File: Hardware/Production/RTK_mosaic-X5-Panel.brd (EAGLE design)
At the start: 151.8 x 101.6 mm, 350 parts, among them J2 MAGJACK-POE, J3 MICRO-SD-PUSH-PUSH-EXT-PIN, J4 Vertical Qwiic Connector, J9 MAGJACK-POE, U1 ESP32-WROVER-IE, U10 POE_PSU-DP990X, U11 SN74AVC4T774PW, U17 URB2405YMD, U2 CH340C, U3 XC6222B331MR-G, U4 TXS0108, U5 TXS0108, U6 XC6222B331MR-G, U7 KSZ8041NL, U8 MOSAIC-X5X5, U9 KSZ8041NL

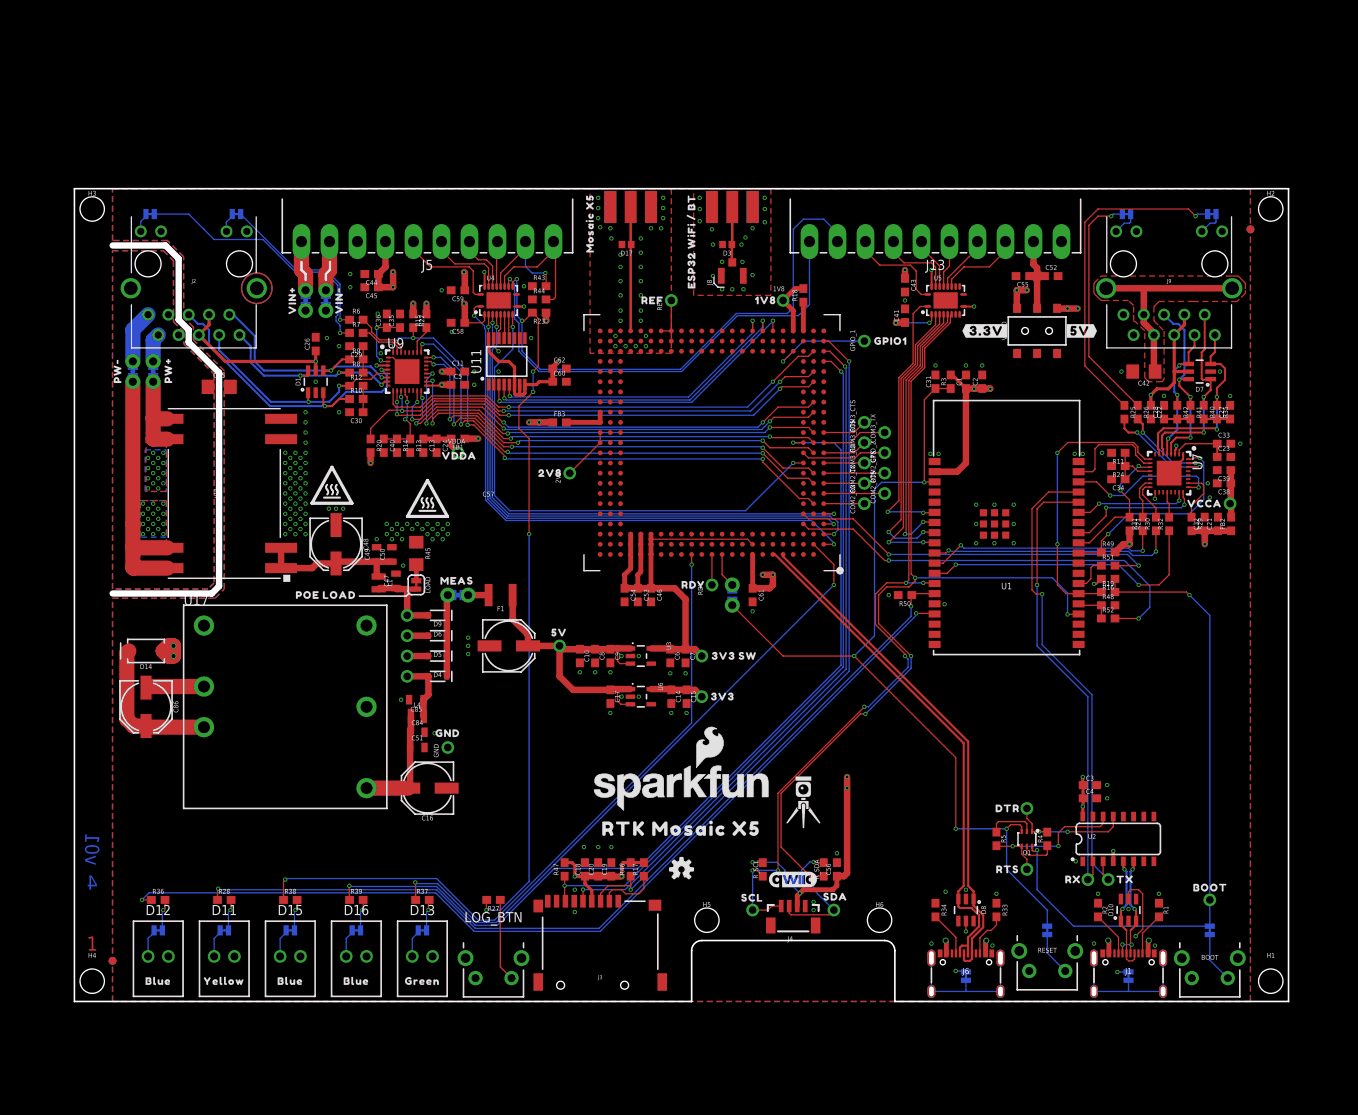
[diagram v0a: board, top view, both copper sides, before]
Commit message: Tweaked and panelized
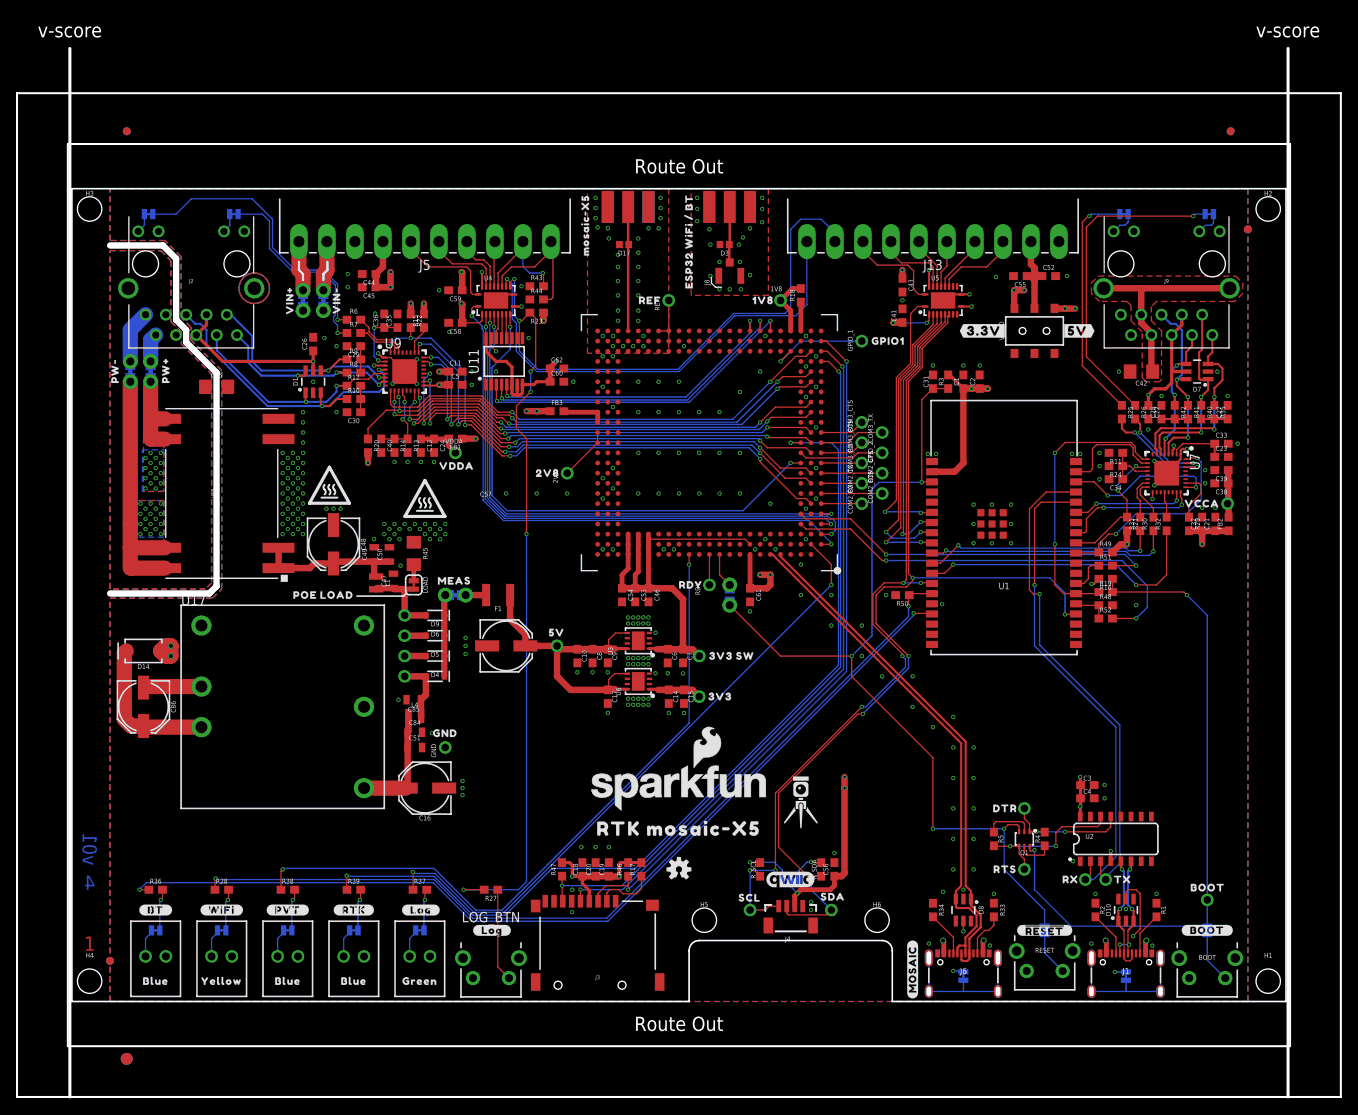
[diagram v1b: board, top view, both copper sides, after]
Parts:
- removed ACT, ACT2: JUMPER-SMT_2_NC_TRACE_SILK, SparkFun-Jumpers:SMT-JUMPER_2_NC_TRACE_SILK
- removed FRAME1: FRAME-LEDGER, SparkFun-Aesthetics:CREATIVE_COMMONS
- removed FRAME3: FRAME-LEDGERNO_FOOTPRINT, SparkFun-Aesthetics:DUMMY
- removed LOGO1: SPECIAL_INSTRUCTIONS-ORDERING, SparkFun-Aesthetics:ORDERING_INSTRUCTIONS
- removed U$100: (no value), output:MOSAIC_X50
- removed U$4: (no value), output:#LINK#1
- removed U$9: (no value), output:#ACT#0
- added E$1, E$2, E$3, E$4: (no value), SparkFun-Aesthetics:FIDUCIAL-1X2
- added E$5, E$6: (no value), SparkFun-Retired:FIDUCIAL-1.5X3
- added SPEED, SPEED2: JUMPER-SMT_2_NC_TRACE_SILK, SparkFun-Jumpers:SMT-JUMPER_2_NC_TRACE_SILK
- added U$109: (no value), output:#_BT_#1
- added U$110, U$116: (no value), output:#_LOG_#5
- added U$111: (no value), output:#_PVT_#3
- added U$112: (no value), output:#_RTK_#4
- added U$115: (no value), output:#_WIFI_#2
- added U$117: (no value), output:#_#RESET#_#0
- added U$118: (no value), output:#_BOOT_#1
- added U$119: (no value), output:#MOSAIC#8
- added U$120: (no value), output:#LINK#1
- added U$121, U$122: (no value), output:#SPEED#0
- U$2: device output:#ACT#0 -> output:MOSAIC#X50
- U$69, U$99: device output:RTK_MOSAIC_X50 -> output:RTK_MOSAIC#X50
- U3, U6: value XC6222B331MR-G -> AP7361C-33FGEUDFN-8; device SparkFun-IC-Power:SOT23-5 -> SparkFun-IC-Power:UDFN-8
- U8: device Septentrio_Mosaic:MOSAIC_LGA -> Septentrio_mosaic-X5:MOSAIC_LGA
- moved U$2 53.5 mm to (64.2, 97.0), flipped to the top, turned to 90 degrees
- moved U$10 11.9 mm to (131.6, 100.1)
- moved LINK 11.0 mm to (131.5, 98.4)
- moved LINK2 11.0 mm to (9.59, 98.4)
- moved U3 1.93 mm to (70.8, 45.1), turned to 90 degrees
- moved U6 1.93 mm to (70.8, 40.0), turned to 90 degrees
- moved FB3 1.43 mm to (60.6, 73.8)
- moved R39 1.31 mm to (35.2, 14.0)
- moved R36 1.31 mm to (10.5, 14.0)
- moved R28 1.31 mm to (18.7, 14.0)
- moved R38 1.31 mm to (27.0, 14.0)
- moved R27 1.31 mm to (52.4, 14.0)
- moved R37 1.31 mm to (43.5, 14.0)
- moved U$97 1.31 mm to (51.0, 66.9)
- moved D10 0.32 mm to (131.8, 11.4)
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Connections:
- net ACT_ESP32 renamed SPEED_ESP32
- net ACT_MOSAIC renamed SPEED_MOSAIC
- net N$13 renamed ESP32_RF
- removed net ACT: ACT.1, J9.14
- removed net ACT2: ACT2.1, J2.14
- removed net LINK: J9.12, LINK.1
- removed net LINK2: J2.12, LINK2.1
- new net N$3: J9.14, LINK.1
- new net N$40: J2.14, LINK2.1
- new net N$41: J2.12, SPEED2.1
- new net N$7: J9.12, SPEED.1
- net 3.3V: now also U6.1; no longer U6.5
- net 3.3V_SW: now also U3.1; no longer U3.5
- net 5V: now also U3.5, U3.8, U6.5, U6.8; no longer U3.1, U3.3, U6.1, U6.3
- net GND: now also U3.4, U3.EP, U6.4, U6.EP; no longer U3.2, U6.2
- net N$12: now also SPEED.2; no longer ACT.2
- net N$142: now also SPEED2.2; no longer ACT2.2
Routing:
- net N$143: track 21.7 -> 36.0 mm
- net N$21: track 41.5 -> 30.1 mm
- net N$12: track 29.8 -> 40.3 mm
- net N$142: track 34.1 -> 25.3 mm
- net GND: track 8.92 -> 17.6 mm, vias 204 -> 330
- net CH340-TXO: track 57.1 -> 60.8 mm
- net N$7: track 0.00 -> 3.32 mm
- net N$3: track 0.00 -> 3.30 mm
- net ACT: track 3.30 -> 0.00 mm
- net LINK: track 3.25 -> 0.00 mm
- net MOSAIC_LOG_BTN_IO: track 148.9 -> 151.7 mm
- net LINK2: track 2.48 -> 0.00 mm
- net N$40: track 0.00 -> 2.48 mm
- net N$41: track 0.00 -> 2.46 mm
- net ACT2: track 2.43 -> 0.00 mm
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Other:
- board size 151.8 x 101.6 mm -> 165.5 x 131.1 mm
- board text added: "Route Out"
- board text added: "v-score"
- board text removed: "Controlled Impedance: JLC7628 Material: TG155 4-Layers Thickness: 1.6mm Outer Copper: 1oz Inner Copper: 0.5oz Finish: ENIG Red Solder Resist White Silkscreen No clean process"
- board text removed: "Dimensions In Inches"
- board text removed: "Paul Clark"
- board text removed: "V-Score To V-Score"
